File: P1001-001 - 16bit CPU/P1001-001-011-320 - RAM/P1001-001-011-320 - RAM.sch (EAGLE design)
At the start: 42 parts, among them IC1 74ALS21D, IC10 74ALS08D, IC2 74283D, IC27 MEGA8535-A, IC3 74ALS04D, IC4 74ALS02D, IC5 74LS32D, IC6 74283D, IC7 74283D, IC8 74283D, IC9 74LS32D

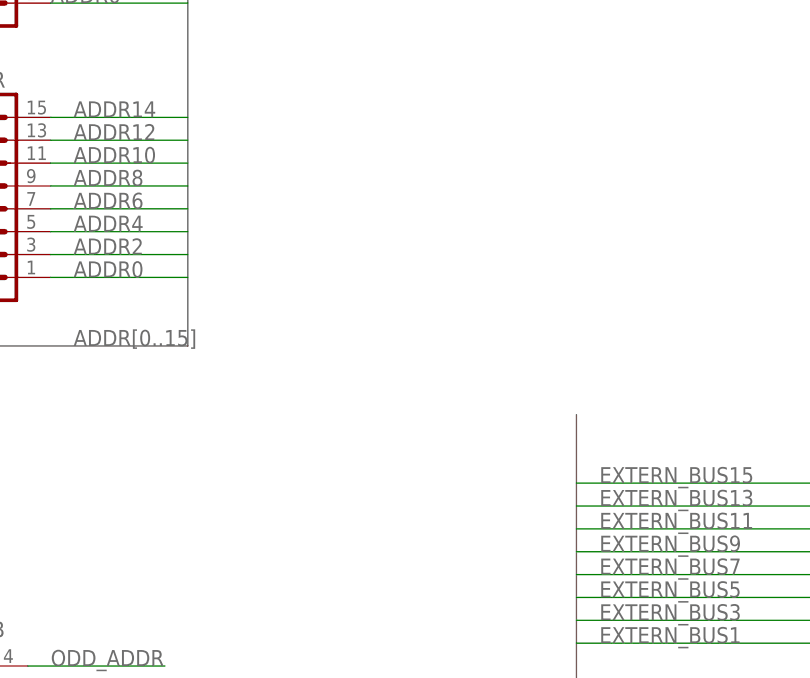
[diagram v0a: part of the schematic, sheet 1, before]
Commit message: Finished All Boards
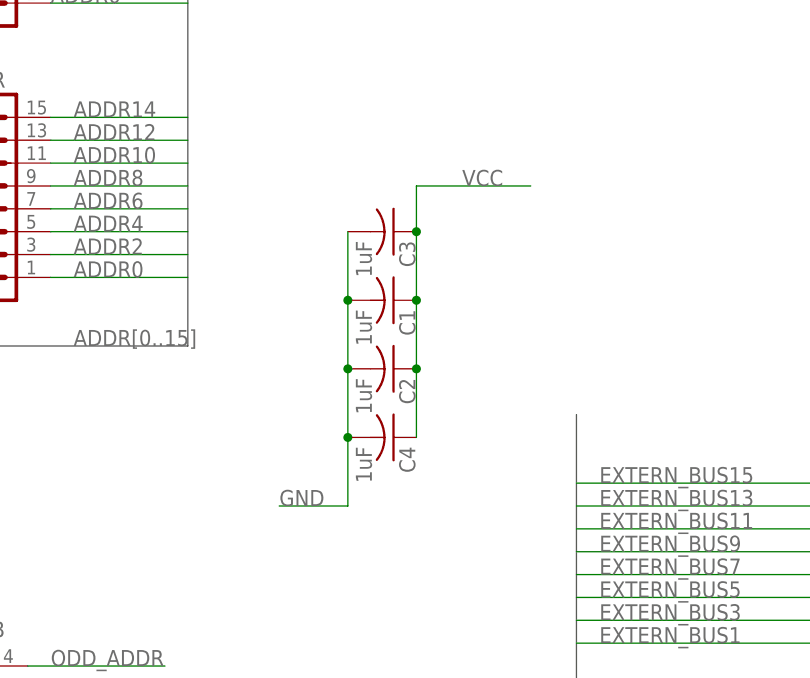
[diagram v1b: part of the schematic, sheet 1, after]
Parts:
- added C1, C2, C3, C4: 1uF, rcl:C-USC1206
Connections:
- net GND: now also C1.2, C2.2, C3.2, C4.2
- net VCC: now also C1.1, C2.1, C3.1, C4.1
